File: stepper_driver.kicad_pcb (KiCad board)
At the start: 4 copper layers, 56 x 56 mm, 83 parts, among them IC1 TMC2160-TA, J1 BARREL_JACK, J2 Screw_Terminal_01x04, J3 CONN_02X07, J4 CONN_01X04, J9 USB_C_Receptacle_USB2.0, Q1 Q_NPN_BEC, Q2 Si4946BEY, Q3 Si4946BEY, Q4 Q_NPN_BEC, Q5 Si4946BEY, Q6 Si4946BEY, SW1 SW_Push, SW2 SW_Push, U1 CH340B, U2 XC6210B332MR, U3 XL1509-5.0, U4 ESP32-WROOM-32D, U6 SN74LV1T34DBV

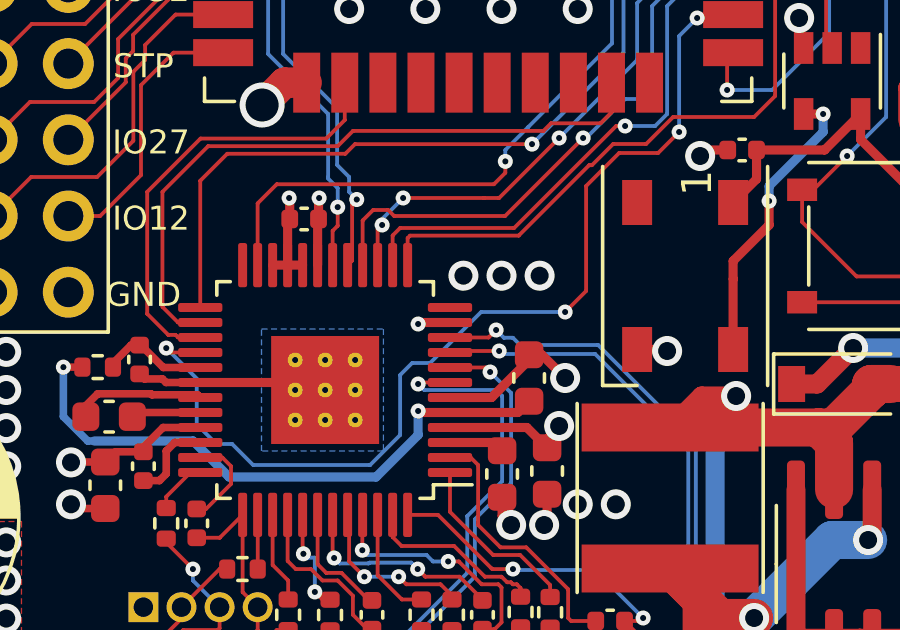
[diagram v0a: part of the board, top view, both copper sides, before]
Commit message: Minor board updates
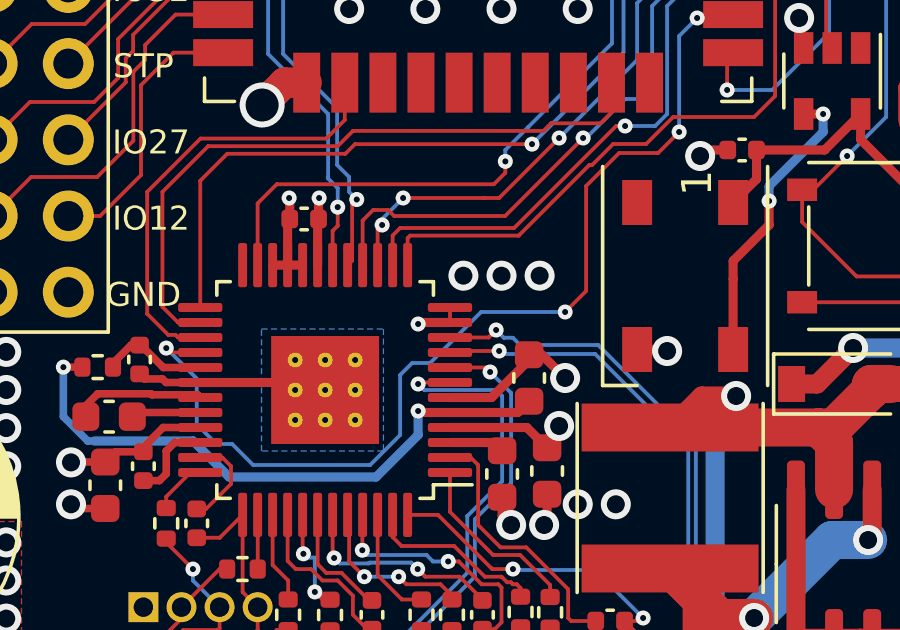
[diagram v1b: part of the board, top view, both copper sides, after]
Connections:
- IC1 pad 12: (no net) -> GND
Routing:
- net GND: track 106.0 -> 106.5 mm
